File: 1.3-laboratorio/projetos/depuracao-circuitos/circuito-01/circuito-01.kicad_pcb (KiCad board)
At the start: 2 copper layers, 73.7 x 52.1 mm, 22 parts, among them J1 Conn_01x07_Male, J2 Conn_01x07_Male, J3 Conn_01x07_Male, J4 Conn_01x07_Male, J5 Conn_01x07_Male, J6 Conn_01x07_Male, J7 Conn_01x04, J8 Conn_01x04, P1 CONN_01X02, SW1 SW_DIP_x04, U1 74LS32, U2 7400, U3 74LS386

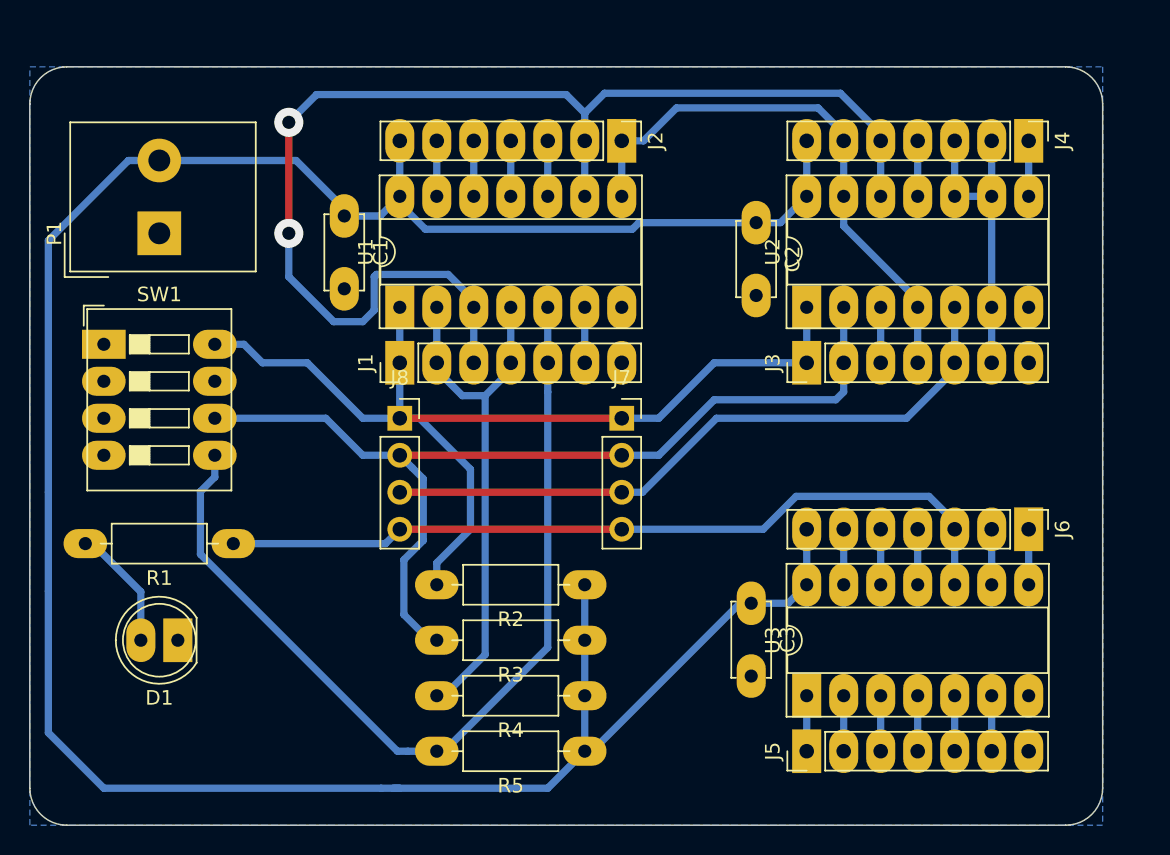
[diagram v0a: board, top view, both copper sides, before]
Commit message: Leiaute quase finalizado para Circuito 01.
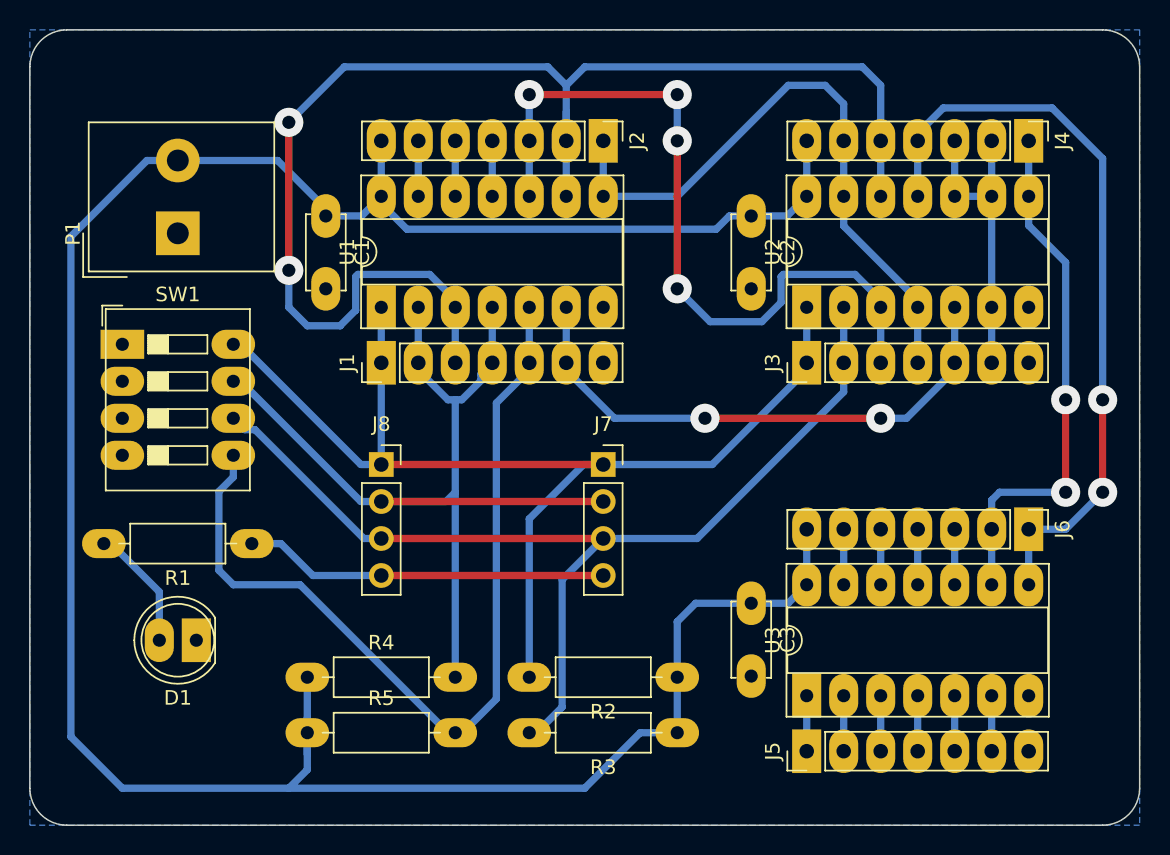
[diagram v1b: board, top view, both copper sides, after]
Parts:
- moved R4 19.1 mm to (157.5, 120.7), turned to 0 degrees
- moved R5 19.1 mm to (157.5, 124.5), turned to 0 degrees
- moved R2 8.98 mm to (182.9, 120.7)
- moved R3 8.98 mm to (182.9, 124.5)
- moved J8 3.42 mm to (162.6, 106.0)
- moved J7 3.42 mm to (177.8, 106.0)
- moved C1 1.27 mm to (158.8, 89.0)
- moved D1 1.27 mm to (149.9, 118.1)
- moved J1 1.27 mm to (162.6, 99.1)
- moved P1 1.27 mm to (148.6, 90.2)
- moved SW1 1.27 mm to (144.8, 97.8)
- moved U1 1.27 mm to (162.6, 95.2)
- moved J2 1.27 mm to (177.8, 83.8)
- moved R1 1.27 mm to (153.7, 111.5)
- moved C2 0.57 mm to (188.0, 89.0)
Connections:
- J7 pad 2: /U2-02 -> /U1-02
- J7 pad 3: /U1-06 -> /U2-02
- J8 pad 2: /U2-02 -> /U1-02
- J8 pad 3: /U1-06 -> /U2-02
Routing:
- net /U1-10: track 7.62 -> 52.8 mm, vias 0 -> 4
- net /U2-11: track 7.62 -> 52.0 mm, vias 0 -> 2
- net /U1-02: track 37.4 -> 68.6 mm
- net /U2-08: track 7.62 -> 36.3 mm, vias 0 -> 2
- net /U3-10: track 55.9 -> 28.8 mm
- net /U1-06: track 50.2 -> 38.0 mm, vias 0 -> 2
- net /U1-03: track 86.6 -> 94.5 mm
- net /U1-01: track 70.9 -> 78.1 mm
- net /U1-08: track 38.6 -> 43.9 mm
- net /U2-02: track 67.0 -> 71.0 mm
- net /U1-05: track 63.0 -> 60.8 mm
- net VCC: track 175.5 -> 177.2 mm
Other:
- board size 73.7 x 52.1 mm -> 76.2 x 54.6 mm
